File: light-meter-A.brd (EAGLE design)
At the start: 56.8 x 55.9 mm, 53 parts, among them IC1 ATMEGA328P, IC2 MCP73831, IC4 MCP1700-33, J1 AYZ0202, J2 AYZ0202, Q4 BSS123, Q5 BSS123, Q6 BSS123, Q7 BSS123, U1 MLX90614_, X1 USBSMD

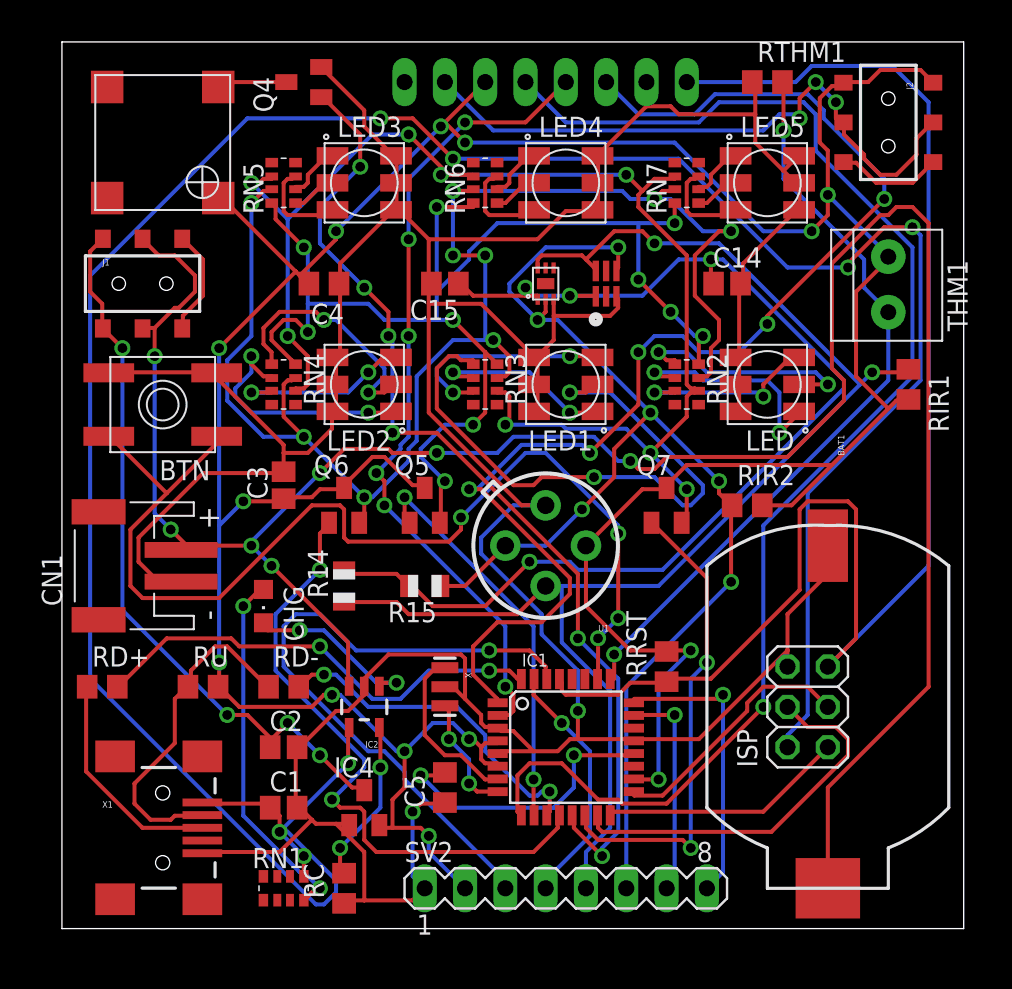
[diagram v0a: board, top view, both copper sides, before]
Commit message: tighter board
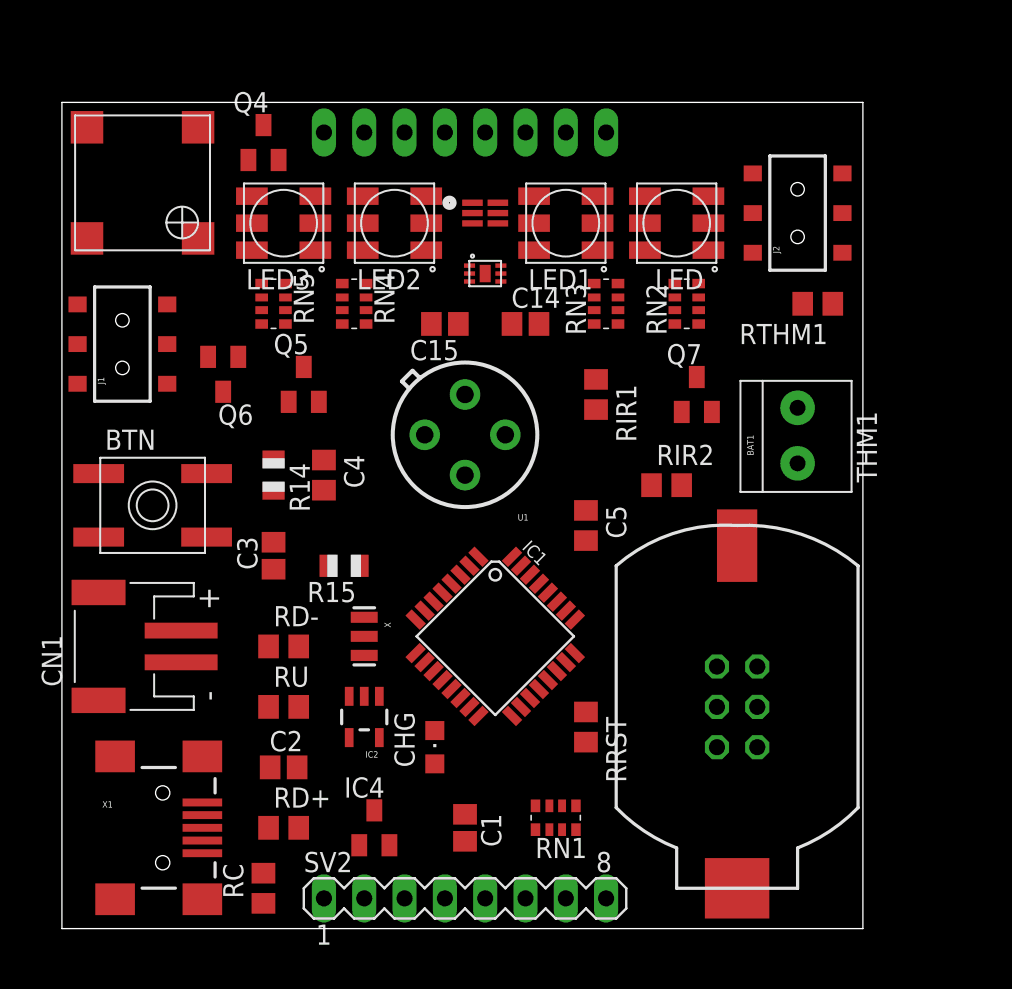
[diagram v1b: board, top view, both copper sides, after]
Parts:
- removed LED4, LED5: RGBLED5050, adafruit:RGBLED5050
- removed RN6, RN7: (no value), resistor-dil:EXB38V
- moved RIR1 19.7 mm to (33.7, 33.7)
- moved C5 18.8 mm to (33.0, 25.4), turned to 270 degrees
- moved RN1 17.7 mm to (31.1, 6.99), turned to 180 degrees
- moved RD+ 14.5 mm to (14.0, 6.35)
- moved RTHM1 14.3 mm to (47.6, 39.4), turned to 180 degrees
- moved CHG 14.0 mm to (23.5, 11.4), turned to 0 degrees
- moved C14 13.0 mm to (29.2, 38.1)
- moved C4 12.1 mm to (16.5, 28.6), turned to 270 degrees
- moved LED 11.7 mm to (38.7, 44.5)
- moved C1 11.5 mm to (25.4, 6.35), turned to 270 degrees
- moved Q6 11.2 mm to (10.2, 34.9), turned to 180 degrees
- moved THM1 11.1 mm to (46.4, 31.1)
- moved Q5 10.8 mm to (15.2, 34.3)
- moved LED2 10.3 mm to (21.0, 44.5)
- moved LED1 10.2 mm to (31.8, 44.5)
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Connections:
- removed net N$21: LED4.3, RN6.3
- removed net N$22: LED4.1, RN6.2
- removed net N$23: LED4.2, RN6.1
- removed net N$24: LED5.3, RN7.3
- removed net N$25: LED5.1, RN7.2
- removed net N$26: LED5.2, RN7.1
- net BLUE: no longer RN6.7, RN7.7
- net GND: now also N1.8; no longer LED4.4, LED4.5, LED4.6, LED5.4, LED5.5, LED5.6
- net GREEN: no longer RN6.6, RN7.6
- net RED: no longer RN6.8, RN7.8
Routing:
- net GND: track 267.8 -> 0.00 mm, vias 2 -> 0
- net VCC: track 218.3 -> 0.00 mm, vias 14 -> 0
- net VBUS: track 168.0 -> 0.00 mm, vias 7 -> 0
- net VBAT: track 145.2 -> 0.00 mm, vias 7 -> 0
- net BLUE: track 96.0 -> 0.00 mm, vias 9 -> 0
- net RESET: track 93.3 -> 0.00 mm
- net SDA: track 90.1 -> 0.00 mm, vias 2 -> 0
- net D5: track 85.9 -> 0.00 mm, vias 1 -> 0
- net GREEN: track 85.8 -> 0.00 mm, vias 8 -> 0
- net RED: track 81.3 -> 0.00 mm, vias 10 -> 0
- net D3: track 81.2 -> 0.00 mm, vias 5 -> 0
- net SCL: track 77.0 -> 0.00 mm, vias 6 -> 0
- net +3V3: track 72.9 -> 0.00 mm, vias 4 -> 0
- net A3: track 67.2 -> 0.00 mm, vias 4 -> 0
- net D9: track 63.2 -> 0.00 mm, vias 6 -> 0
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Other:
- board size 56.8 x 55.9 mm -> 50.5 x 52.1 mm
